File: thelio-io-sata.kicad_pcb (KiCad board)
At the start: 2 copper layers, 80.2 x 71.8 mm, 6 parts

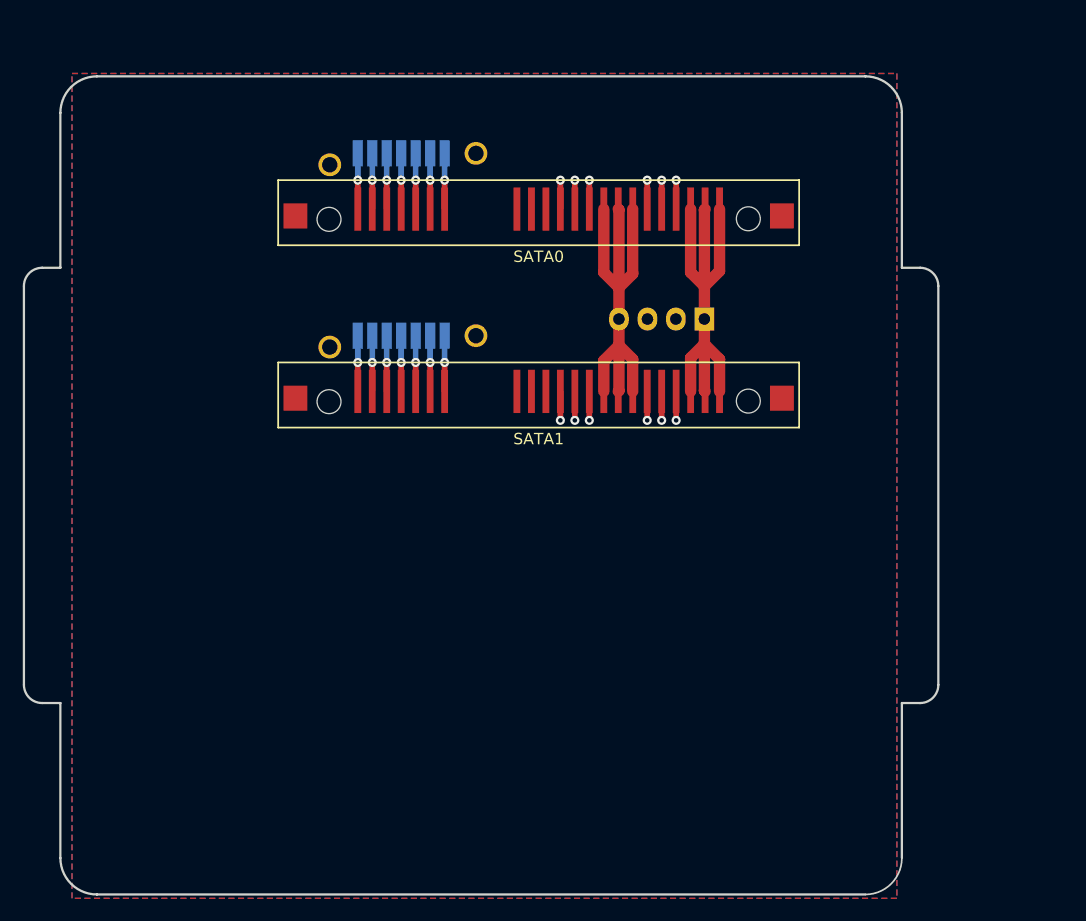
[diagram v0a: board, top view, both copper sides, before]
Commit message: Update SATA design
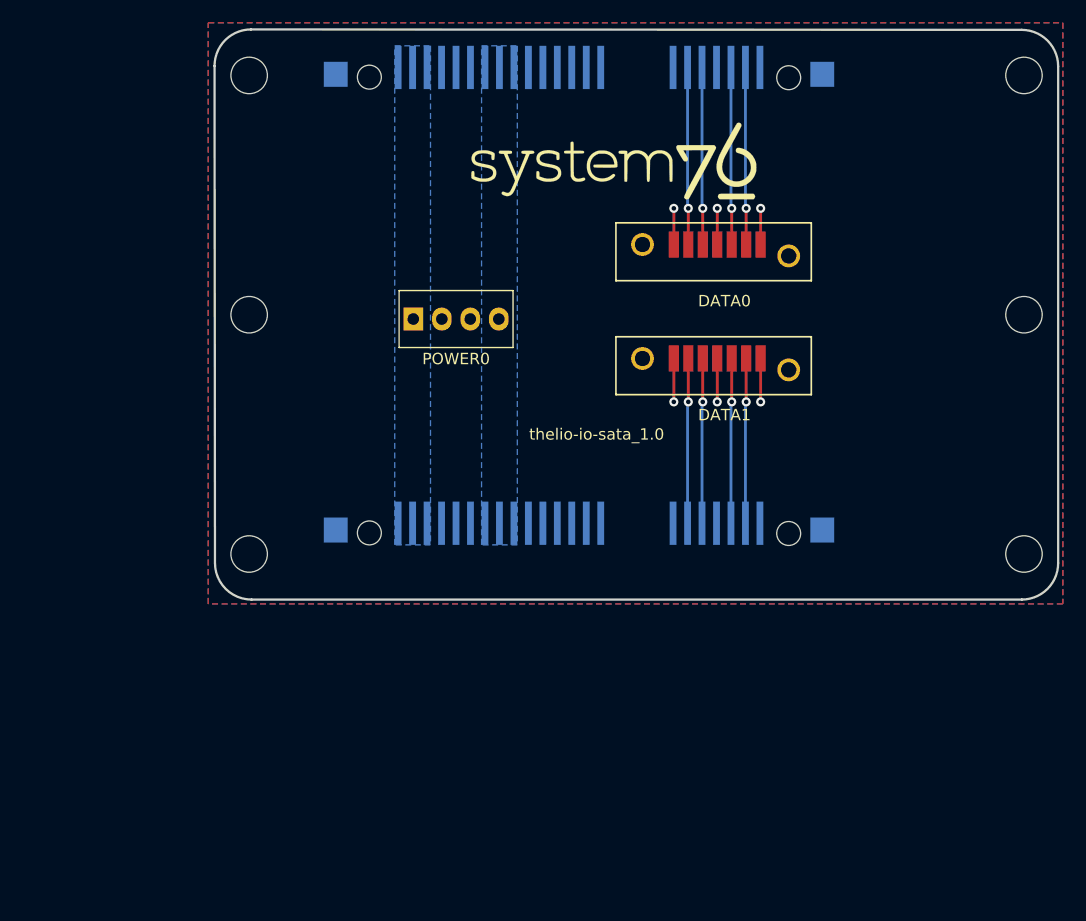
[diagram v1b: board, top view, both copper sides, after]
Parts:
- added REF**: MountingHole_3.2mm_M3, MountingHole:MountingHole_3.2mm_M3, F.Cu at (116.6, 73.9)
- added REF**: MountingHole_3.2mm_M3, MountingHole:MountingHole_3.2mm_M3, F.Cu at (48.6, 73.9)
- added REF**: MountingHole_3.2mm_M3, MountingHole:MountingHole_3.2mm_M3, F.Cu at (48.6, 52.9)
- added REF**: MountingHole_3.2mm_M3, MountingHole:MountingHole_3.2mm_M3, F.Cu at (116.6, 52.9)
- added REF**: MountingHole_3.2mm_M3, MountingHole:MountingHole_3.2mm_M3, F.Cu at (48.6, 31.9)
- added REF**: MountingHole_3.2mm_M3, MountingHole:MountingHole_3.2mm_M3, F.Cu at (116.6, 31.9)
- DATA0, DATA1, G***, POWER0: moved to F.Cu
- SATA0, SATA1: moved to B.Cu
- moved DATA0 30.1 mm to (90.3, 44.2), turned to 0 degrees
- moved DATA1 29.1 mm to (90.3, 54.2), turned to 0 degrees
- moved POWER0 18.0 mm to (66.7, 53.3), turned to 0 degrees
- moved SATA0 12.9 mm to (77.5, 31.2), turned to 180 degrees
- moved SATA1 12.1 mm to (77.5, 71.2), turned to 180 degrees
- moved G*** 7.71 mm to (80.6, 39.4), turned to 0 degrees
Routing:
- net +5V: track 40.7 -> 0.00 mm
- net +12V: track 40.0 -> 0.00 mm
- net GND: track 59.8 -> 21.0 mm, vias 18 -> 6
- net Net-(DATA0-Pad3): track 4.89 -> 15.6 mm
- net Net-(DATA0-Pad6): track 4.89 -> 15.6 mm
- net Net-(DATA0-Pad5): track 4.89 -> 15.6 mm
- net Net-(DATA0-Pad2): track 4.89 -> 15.6 mm
- net Net-(DATA1-Pad3): track 4.89 -> 14.5 mm
- net Net-(DATA1-Pad6): track 4.89 -> 14.5 mm
- net Net-(DATA1-Pad5): track 4.89 -> 14.5 mm
- net Net-(DATA1-Pad2): track 4.89 -> 14.5 mm
- added copper zone on B.Cu, net +12V
- added copper zone on B.Cu, net +5V
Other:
- board size 80.2 x 71.8 mm -> 74 x 50 mm
- board text added: "thelio-io-sata_1.0"
